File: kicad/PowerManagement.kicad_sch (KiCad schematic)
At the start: 42 parts, among them U13 AMS1117-3.3, U3 MP9488GS-Z, U5 AP63205, U56 MCP1416, U57 IRF644SPBF, U58 STEF4S, U59 STEF4S

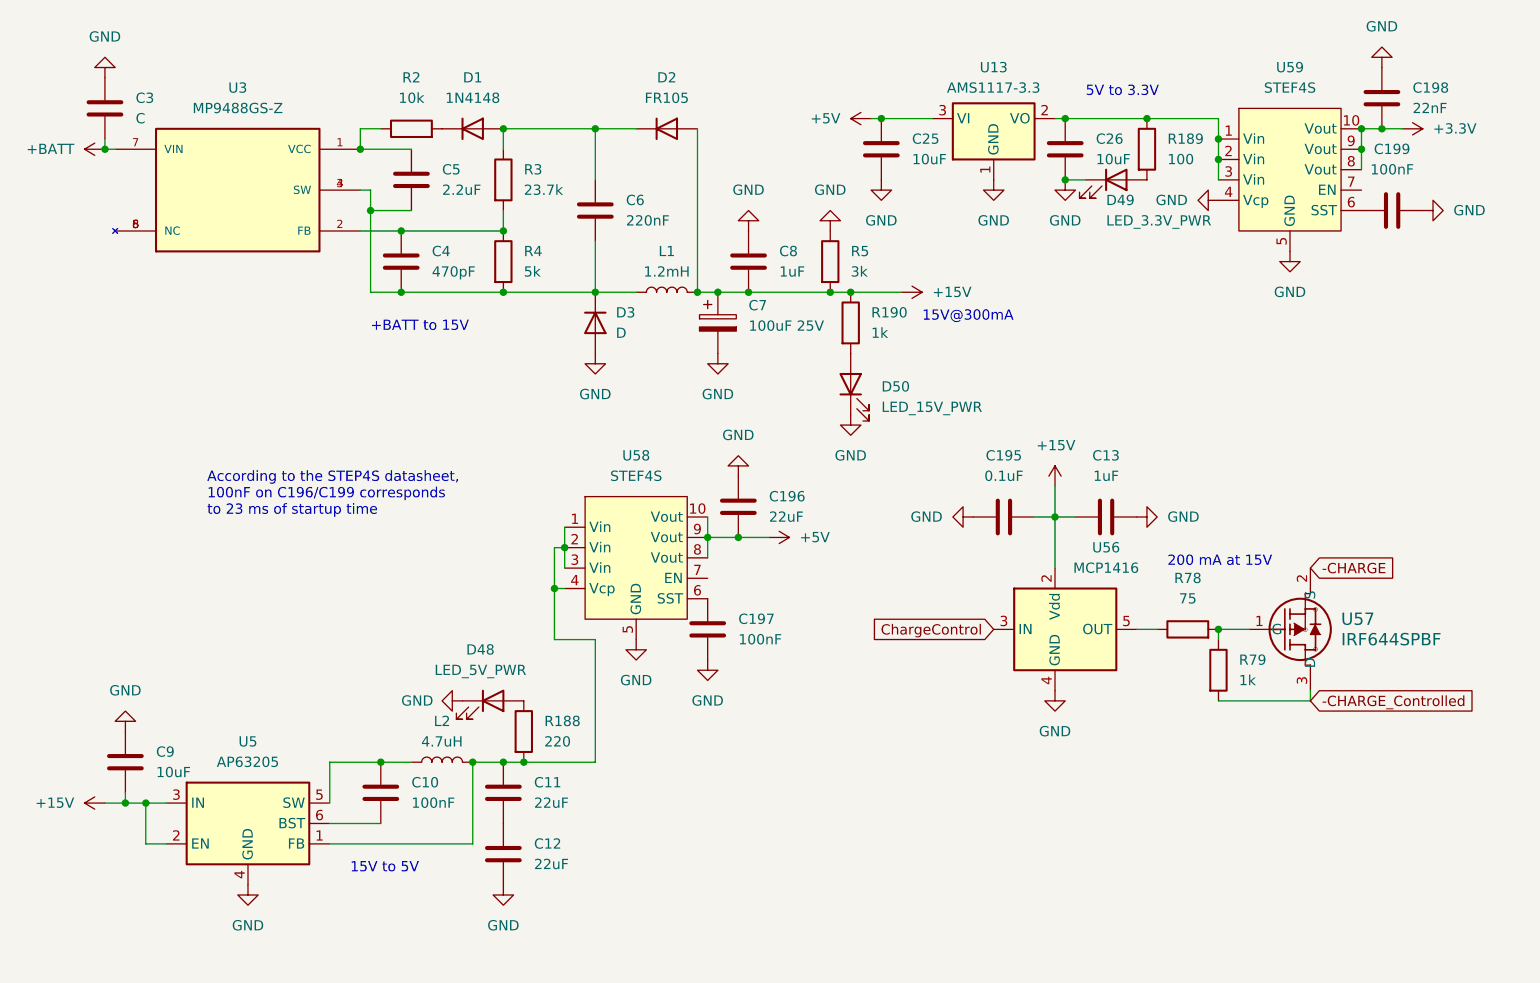
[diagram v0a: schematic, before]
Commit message: Finished SBMS-T-3, started work on SBMS-T-4
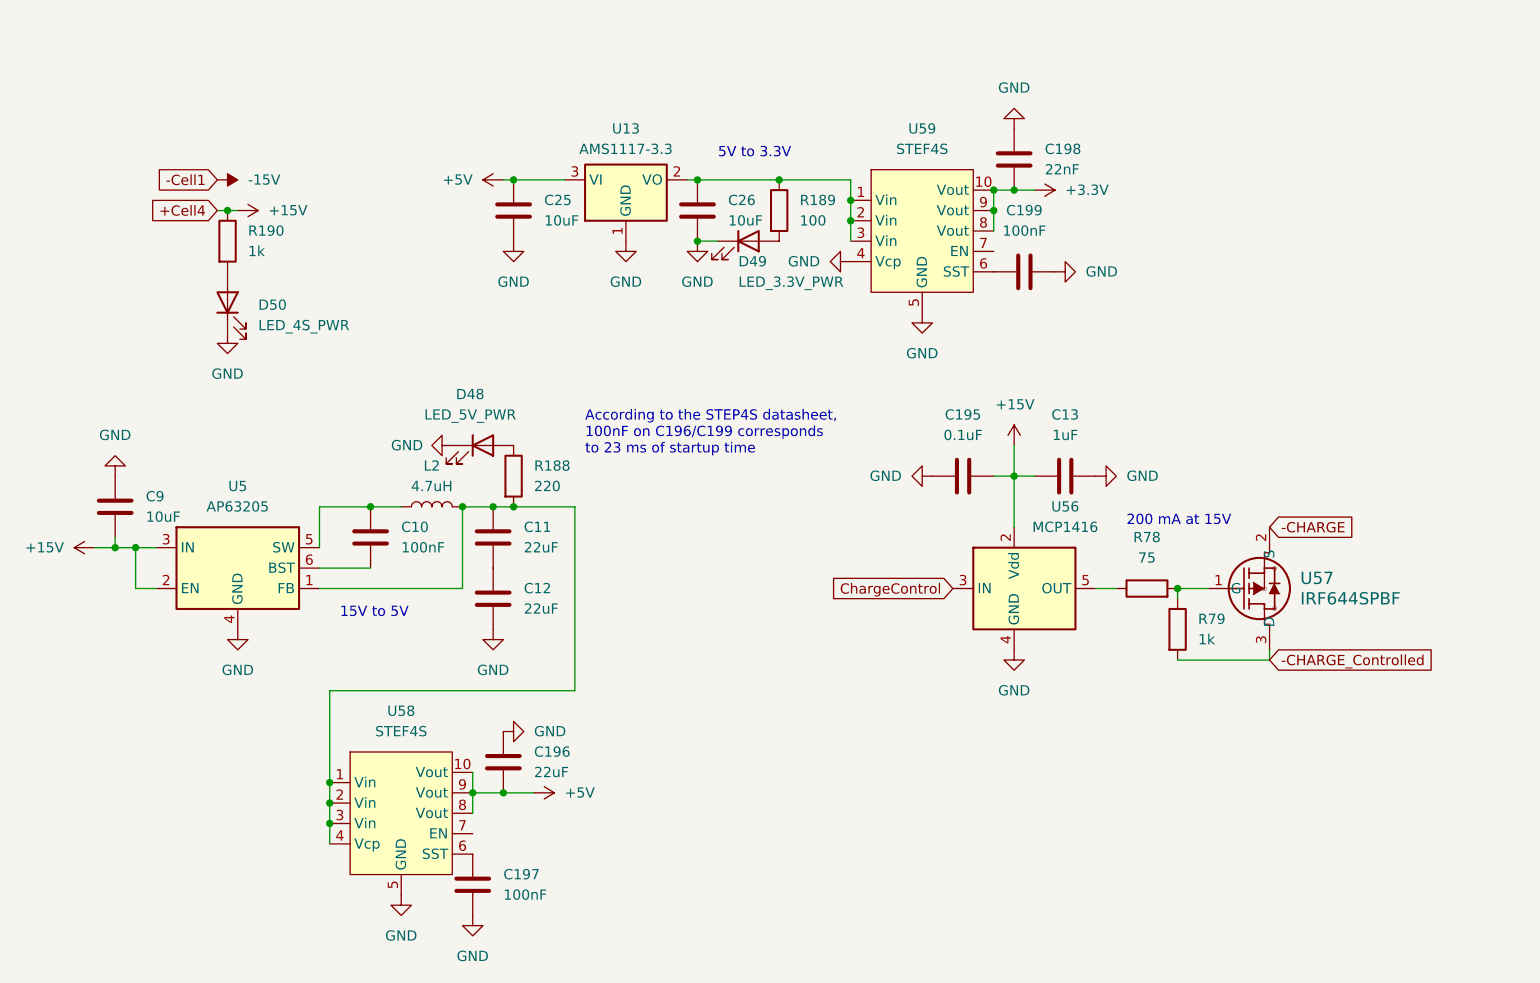
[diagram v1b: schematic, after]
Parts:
- removed C3: C, symbol Device:C
- removed C4: 470pF, symbol Device:C
- removed C5: 2.2uF, symbol Device:C
- removed C6: 220nF, symbol Device:C
- removed C7: 100uF 25V, symbol Device:C_Polarized
- removed C8: 1uF, symbol Device:C
- removed D1: 1N4148, symbol Device:D
- removed D2: FR105, symbol Device:D
- removed D3: D, symbol Device:D
- removed L1: 1.2mH, symbol Device:L
- removed R2: 10k, symbol Device:R
- removed R3: 23.7k, symbol Device:R
- removed R4: 5k, symbol Device:R
- removed R5: 3k, symbol Device:R
- removed U3: MP9488GS-Z, MP9488GS-Z:SOIC127P600X175-8N, symbol MP9488GS-Z:MP9488GS-Z
- D50: value LED_15V_PWR -> LED_4S_PWR
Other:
- note removed: "+BATT to 15V"
- note removed: "15V@300mA"
- moved on the sheet: C10, C11, C12, C13, C195, C196, C197, C198, C199, C25, C26, C9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
